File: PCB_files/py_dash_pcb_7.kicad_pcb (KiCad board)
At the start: 4 copper layers, 203.8 x 102.4 mm, 104 parts, among them J1 FFC2B28-40-G, J2 CANbus, J5 Micro_SD_Card_Det1, J8 USB_C_Receptacle_USB2.0_14P, Q1 DMG2307, Q2 DMG2307, Q3 DMG2307, SW1 SW_Push, SW2 SW_Push, SW3 SW_Push, SW4 SW_Push, SW5 SW_Push, SW6 SW_Push, SW7 nBoot, U1 CM4102008, U10 EMIF06-MSD02N16, U3 AP64501SP-13, U4 TPD8S009DSMR, U5 TPD8S009DSMR, U6 TPD2EUSB30, U7 SN65HVD234, U8 MCP2515-xST, U9 BD33FC0FP, Y1 16Mhz

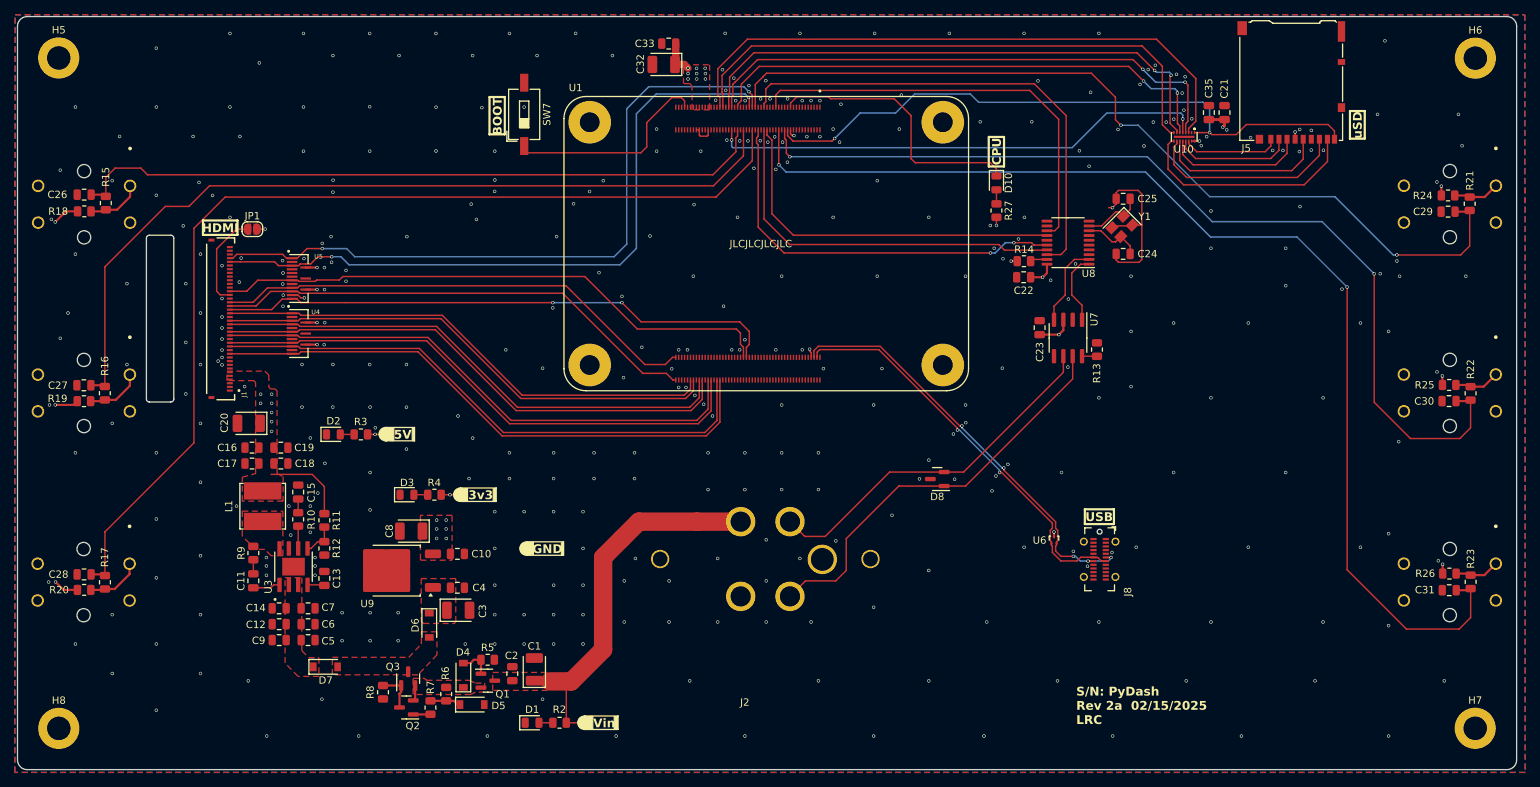
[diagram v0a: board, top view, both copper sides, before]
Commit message: push from desktop to align files
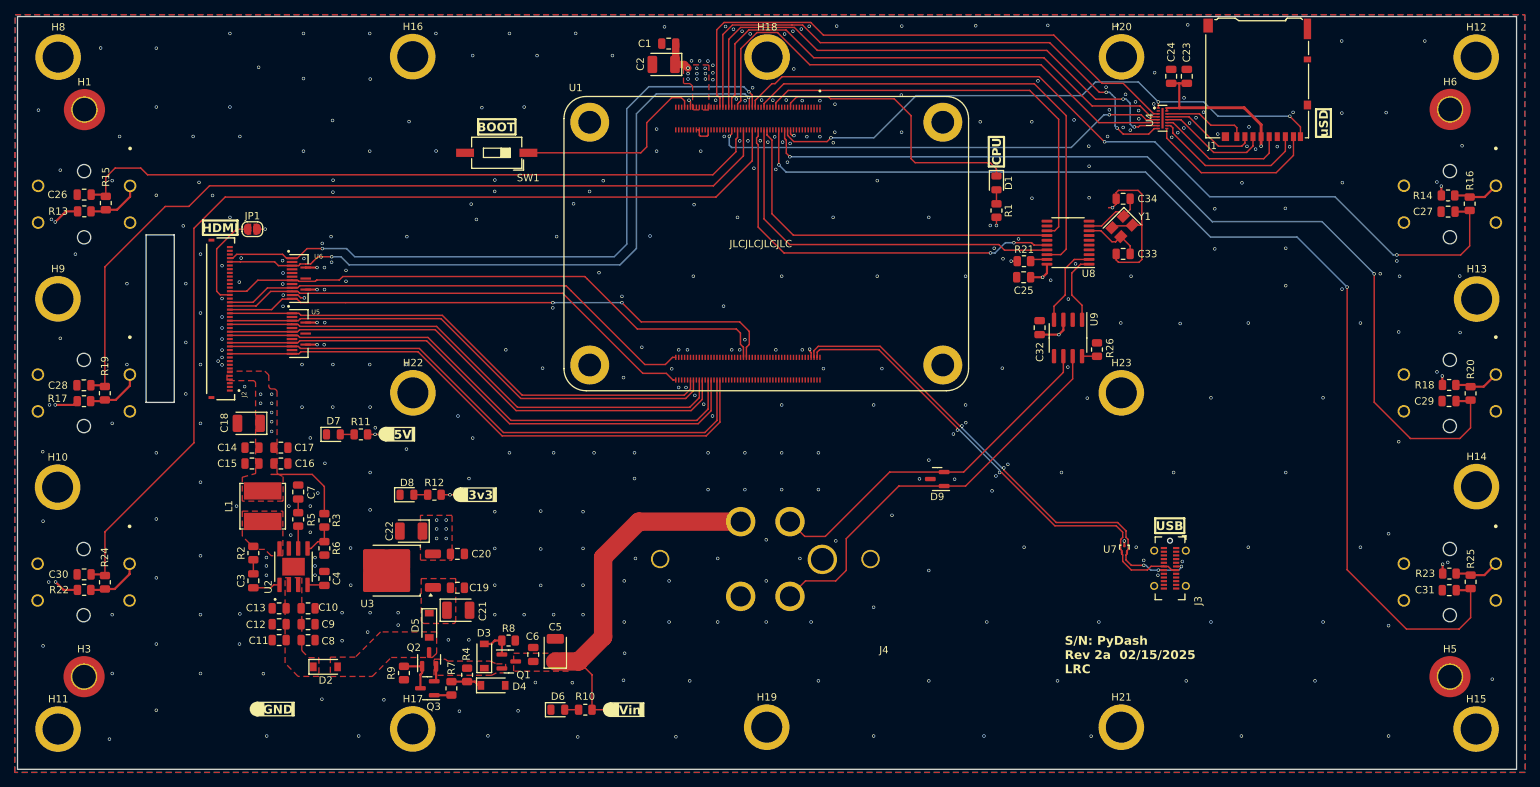
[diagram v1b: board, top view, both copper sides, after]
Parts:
- removed H7: MountingHole, MountingHole:MountingHole_3.2mm_M3_DIN965_Pad
- added H1: MountingHole_M2, MountingHole:MountingHole_3.2mm_M3_DIN965_Pad_TopOnly, F.Cu at (60.2, 57.4)
- added H10: Standoff_M2.5_5ET, user:Standoff_M2.5_5ET, F.Cu at (56.6, 108.7)
- added H11: Standoff_M2.5_5ET, user:Standoff_M2.5_5ET, F.Cu at (56.6, 141.6)
- added H12: Standoff_M2.5_5ET, user:Standoff_M2.5_5ET, F.Cu at (249.4, 50.2)
- added H13: Standoff_M2.5_5ET, user:Standoff_M2.5_5ET, F.Cu at (249.5, 83.1)
- added H14: Standoff_M2.5_5ET, user:Standoff_M2.5_5ET, F.Cu at (249.4, 108.6)
- added H15: Standoff_M2.5_5ET, user:Standoff_M2.5_5ET, F.Cu at (249.4, 141.6)
- added H16: Standoff_M2.5_5ET, user:Standoff_M2.5_5ET, F.Cu at (104.8, 50.1)
- added H17: Standoff_M2.5_5ET, user:Standoff_M2.5_5ET, F.Cu at (104.8, 141.5)
- added H18: Standoff_M2.5_5ET, user:Standoff_M2.5_5ET, F.Cu at (153.0, 50.2)
- added H19: Standoff_M2.5_5ET, user:Standoff_M2.5_5ET, F.Cu at (153.0, 141.3)
- added H20: Standoff_M2.5_5ET, user:Standoff_M2.5_5ET, F.Cu at (201.2, 50.2)
- added H21: Standoff_M2.5_5ET, user:Standoff_M2.5_5ET, F.Cu at (201.2, 141.3)
- added H22: Standoff_M2.5_5ET, user:Standoff_M2.5_5ET, F.Cu at (104.9, 95.8)
- added H23: Standoff_M2.5_5ET, user:Standoff_M2.5_5ET, F.Cu at (201.2, 95.8)
- added H3: MountingHole_M2, MountingHole:MountingHole_3.2mm_M3_DIN965_Pad_TopOnly, F.Cu at (60.2, 134.4)
- added H9: Standoff_M2.5_5ET, user:Standoff_M2.5_5ET, F.Cu at (56.6, 83.1)
- H5, H6: value MountingHole -> MountingHole_M2; footprint MountingHole:MountingHole_3.2mm_M3_DIN965_Pad -> MountingHole:MountingHole_3.2mm_M3_DIN965_Pad_TopOnly
- H8: value MountingHole -> Standoff_M2.5_5ET; footprint MountingHole:MountingHole_3.2mm_M3_DIN965_Pad -> user:Standoff_M2.5_5ET
- moved H5 207.0 mm to (245.8, 134.4)
- moved H8 91.3 mm to (56.6, 50.2)
- moved TP4 42.6 mm to (83.7, 138.8)
- moved J3 9.65 mm to (207.8, 119.7)
- moved U7 9.65 mm to (201.6, 117.1)
- moved H6 7.77 mm to (245.9, 57.3)
- moved C23 7.11 mm to (210.1, 52.8)
- moved C24 7.11 mm to (207.9, 52.8)
- moved SW1 6.42 mm to (116.3, 63.2), turned to 180 degrees
- moved J1 4.64 mm to (219.7, 53.3)
- moved D6 3.92 mm to (124.6, 138.9)
- moved R10 3.92 mm to (128.3, 138.9)
- moved TP3 3.92 mm to (131.7, 138.9)
- moved U4 3.92 mm to (206.6, 58.5), turned to -90 degrees
- moved D3 3.86 mm to (114.6, 131.6)
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- renumbered C33 to C1, C7 to C10, C9 to C11, C14 to C13, C16 to C14, C17 to C15, C18 to C16, C19 to C17, C20 to C18, C4 to C19, C32 to C2, C10 to C20, C3 to C21, C8 to C22, C21 to C23, C35 to C24, C22 to C25, C29 to C27, C27 to C28, C30 to C29, C11 to C3, C28 to C30, C23 to C32, C24 to C33, C25 to C34, C13 to C4, C1 to C5, C2 to C6, C15 to C7, C5 to C8, C6 to C9, D10 to D1, D7 to D2, D4 to D3, D5 to D4, D6 to D5, D1 to D6, D2 to D7, D3 to D8, D8 to D9, J5 to J1, J1 to J2, J8 to J3, J2 to J4, Q3 to Q2, Q2 to Q3, R27 to R1, R2 to R10, R3 to R11, R4 to R12, R18 to R13, R24 to R14, R21 to R16, R19 to R17, R25 to R18, R16 to R19, R9 to R2, R22 to R20, R14 to R21, R20 to R22, R26 to R23, R17 to R24, R23 to R25, R13 to R26, R11 to R3, R6 to R4, R10 to R5, R12 to R6, R5 to R8, R8 to R9, SW7 to SW1, SW4 to SW2, SW1 to SW3, SW5 to SW4, SW2 to SW5, SW3 to SW7, TP4 to TP1, TP1 to TP2, TP2 to TP3, TP3 to TP4, U3 to U2, U9 to U3, U10 to U4, U4 to U5, U5 to U6, U6 to U7, U7 to U9
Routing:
- net +3.3V: track 350.5 -> 364.2 mm, vias 24 -> 22
- net ext_USBD+: track 58.3 -> 68.3 mm
- net ext_USBD-: track 55.3 -> 65.4 mm
- net SD_DET: track 86.4 -> 78.9 mm, vias 2 -> 3
- net Net-(J1-DAT1): track 31.3 -> 24.0 mm
- net Net-(J1-DAT0): track 27.3 -> 21.6 mm
- net SD_DAT2: track 82.0 -> 76.3 mm
- net SD_CMD: track 68.1 -> 62.8 mm
- net Net-(J1-CLK): track 23.3 -> 18.5 mm
- net Net-(J1-CMD): track 19.1 -> 15.2 mm
- net btn_L1: track 120.3 -> 116.8 mm
- net Net-(J1-DAT3/CD): track 16.2 -> 13.3 mm
- net SD_DAT3: track 74.5 -> 72.0 mm, vias 2 -> 0
- net Net-(J1-DAT2): track 13.2 -> 11.5 mm
- net GND: track 4.85 -> 6.40 mm, vias 379 -> 400
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- added copper zone on F.Cu, net Net-(D4-K)
- removed copper zone on F.Cu, net Net-(D3-K)
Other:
- board size 203.8 x 102.4 mm -> 203.8 x 102.3 mm
